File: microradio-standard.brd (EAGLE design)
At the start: 96.5 x 64.4 mm, 13 parts, among them T1 NPN (ECB)

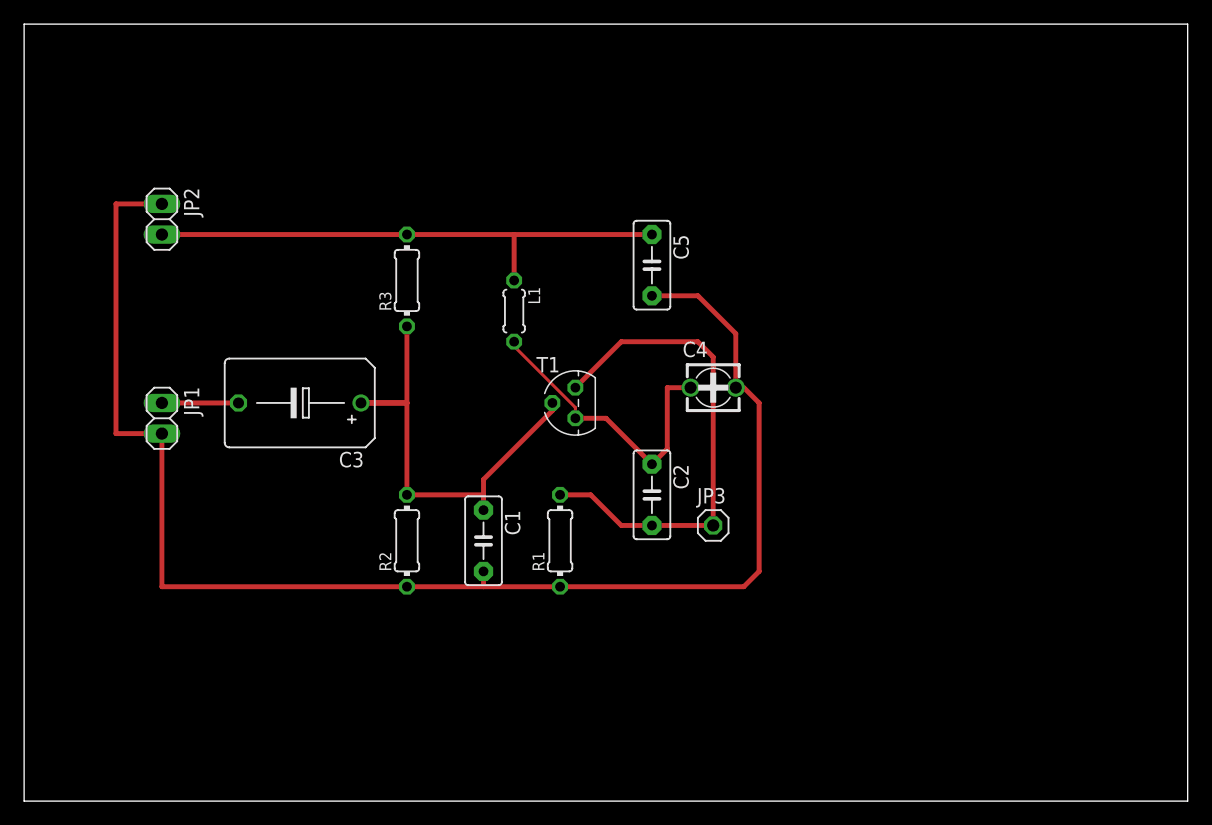
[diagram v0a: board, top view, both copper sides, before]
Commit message: added lib
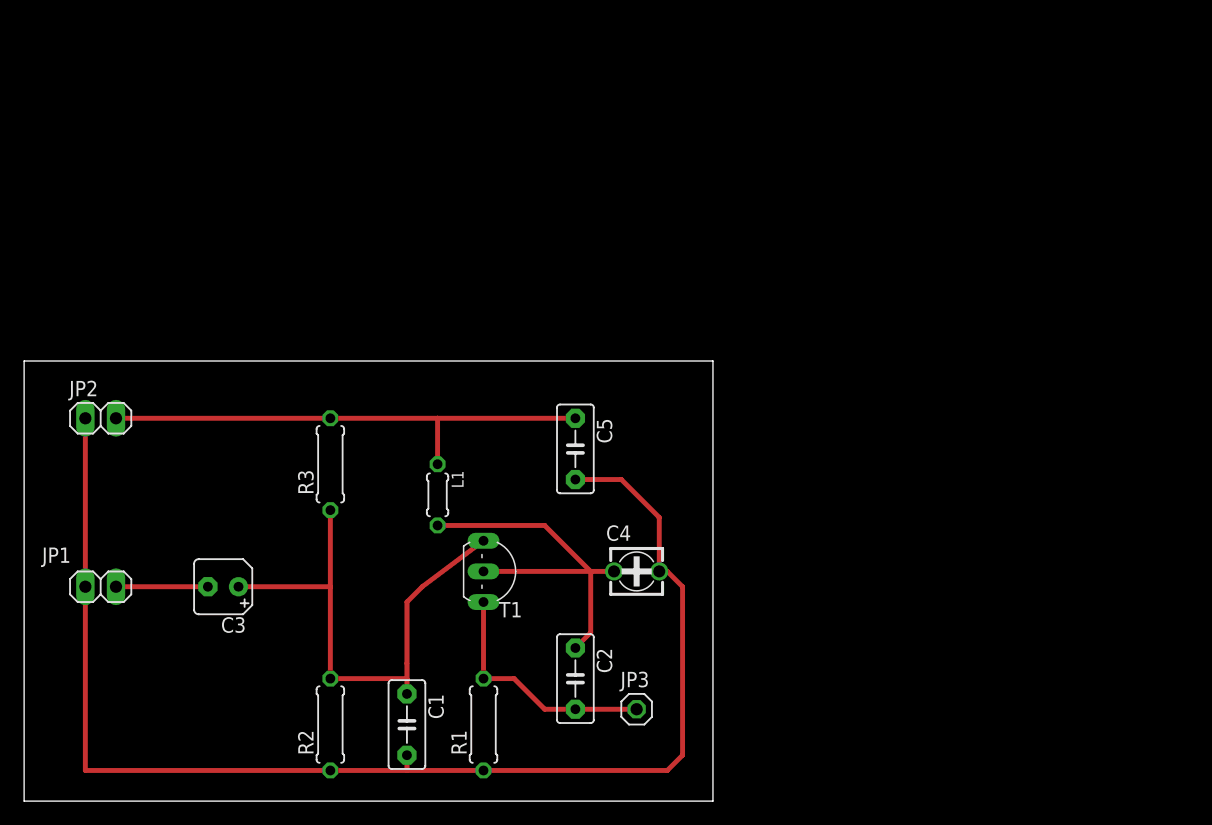
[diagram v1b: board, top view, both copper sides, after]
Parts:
- C1, C2, C5: device capacitor-wima:C5B3 -> microradio-standard:C5B3
- C3: device rcl:B45181C -> microradio-standard:B45181A
- C4: device c-trimm:3008 -> microradio-standard:3008
- JP1, JP2: device pinhead:1X02 -> microradio-standard:1X02
- JP3: device pinhead:1X01 -> microradio-standard:1X01
- L1: device rcl:0204/5 -> microradio-standard:0204/5
- R1, R2, R3: device resistor:0204/7 -> microradio-standard:0207/7
- T1: device transistor:TO92 -> microradio-standard:TO92-BCE
- moved JP2 17.3 mm to (6.35, 31.8), turned to 0 degrees
- moved C3 16.5 mm to (16.5, 17.8)
- moved C5 16.5 mm to (45.7, 29.2)
- moved L1 16.5 mm to (34.3, 25.4)
- moved C1 16.5 mm to (31.8, 6.35)
- moved C2 16.5 mm to (45.7, 10.2)
- moved C4 16.5 mm to (50.8, 19.1)
- moved JP3 16.5 mm to (50.8, 7.62)
- moved R1 16.5 mm to (38.1, 6.35)
- moved R2 16.5 mm to (25.4, 6.35)
- moved R3 16.5 mm to (25.4, 27.9)
- moved T1 15.9 mm to (38.1, 19.1), turned to 270 degrees
- moved JP1 14.9 mm to (6.35, 17.8), turned to 180 degrees
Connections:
- net N$2: now also T1.E; no longer T1.1
- net N$4: now also T1.B; no longer T1.2
- net N$5: now also T1.C; no longer T1.3
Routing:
- net N$2: track 41.3 -> 20.1 mm
- net GND: track 119.9 -> 109.7 mm
- net N$5: track 25.2 -> 32.0 mm
- net N$4: track 40.5 -> 43.7 mm
- net N$3: track 44.5 -> 41.9 mm
- net N$1: track 6.35 -> 7.62 mm
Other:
- board size 96.5 x 64.4 mm -> 57.1 x 36.5 mm
